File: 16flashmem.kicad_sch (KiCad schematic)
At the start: 9 parts, among them IC1 MX25V1635FZNQ03-T

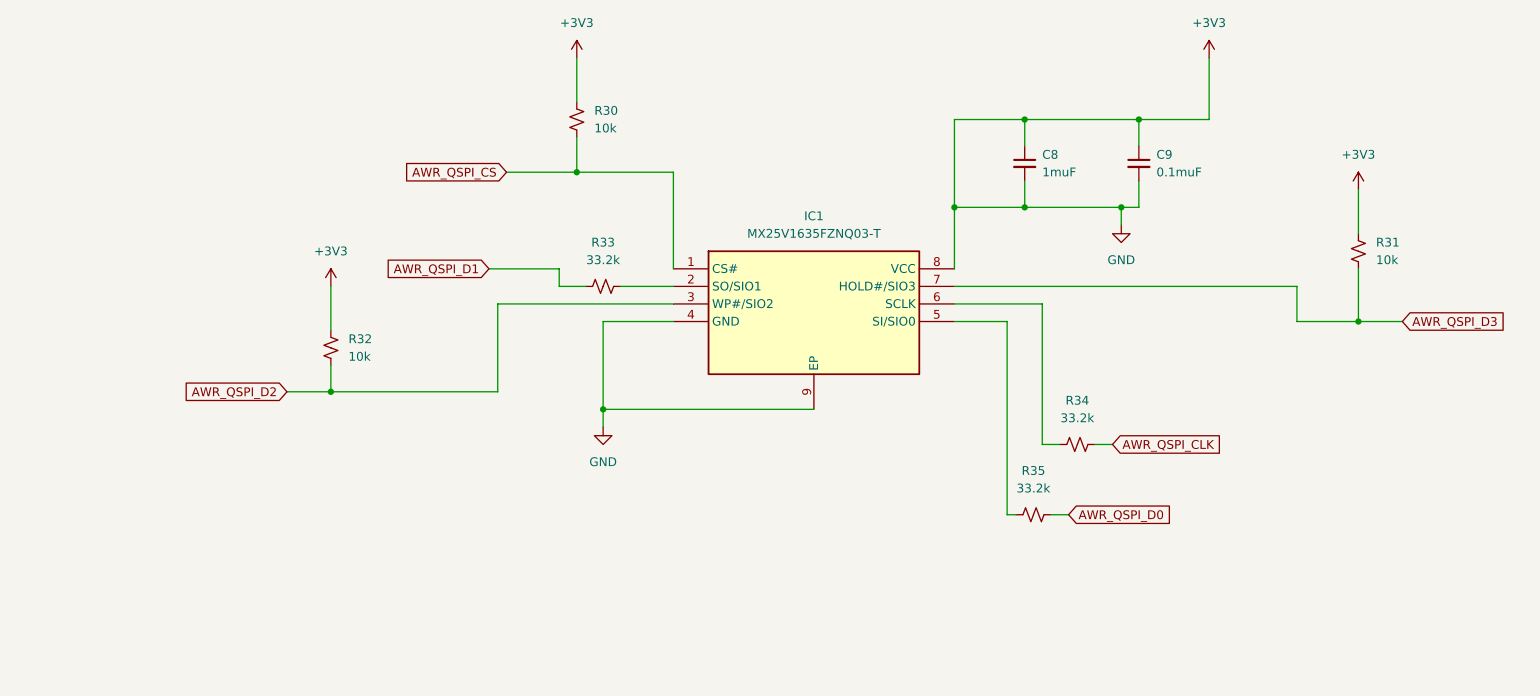
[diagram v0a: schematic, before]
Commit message: decoup and lc schematics
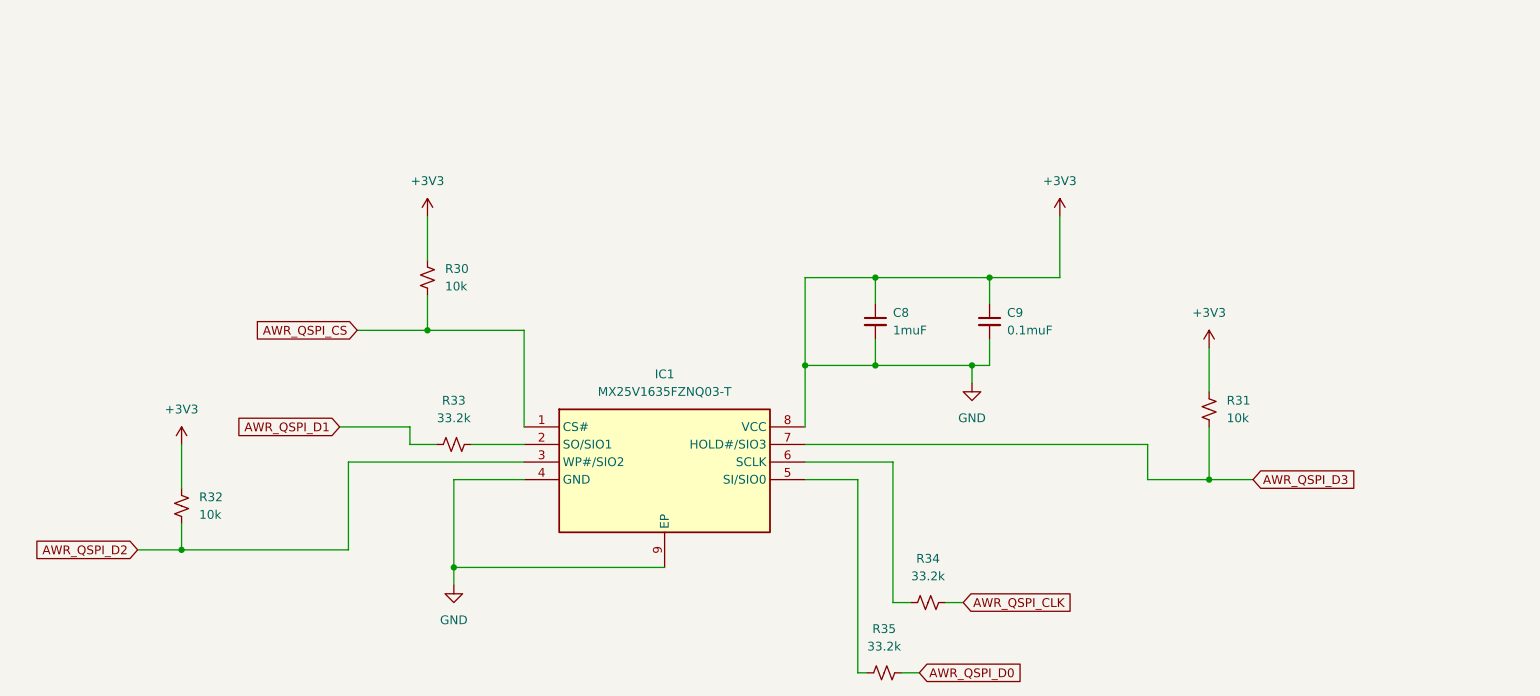
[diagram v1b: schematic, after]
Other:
- moved on the sheet: C8, C9, IC1, R30, R31, R32, R33, R34, R35
